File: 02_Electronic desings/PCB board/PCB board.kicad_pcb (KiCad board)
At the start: 2 copper layers, 131.6 x 84.8 mm, 31 parts, among them J10 Switch Manual/Auto, J11 Jetson, J12 Compass, J15 M2_Controll, J16 Power +5V, J17 GPS, J18 Power +5V, J19 Power +5V, J20 I2C, J21 Power +5V, J22 XBee, J3 Power +5V, J4 M1 encoder, J5 PS2_Controll, J6 M2 encoder, J8 Arduino_Mega_Header, J9 M1_Controll, U3 Logic_Level_Converter, U4 Screw_term_p2_5mm

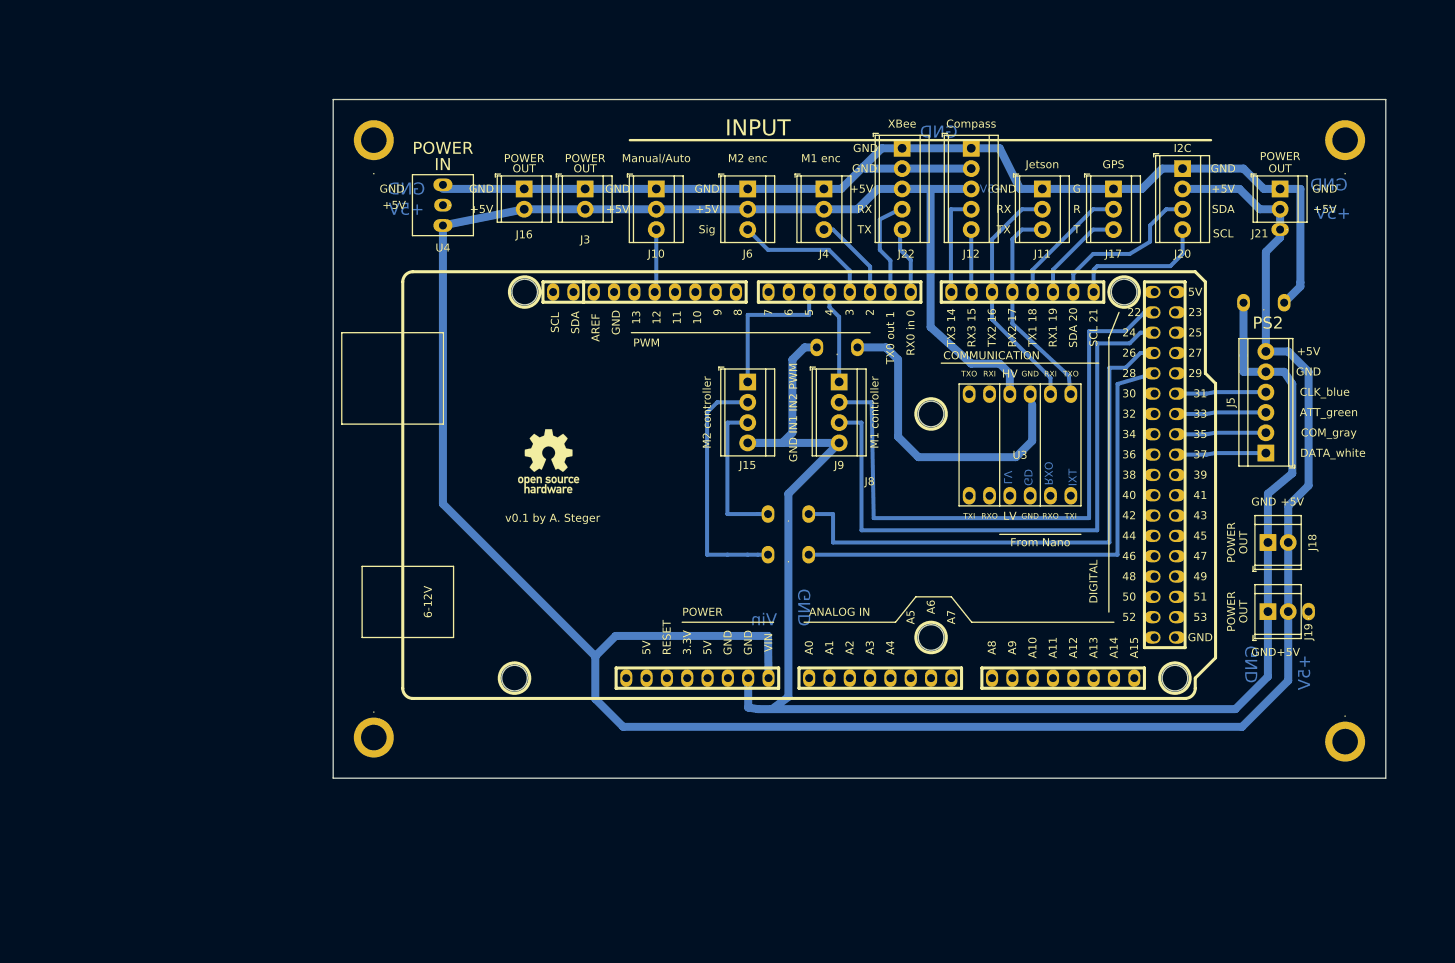
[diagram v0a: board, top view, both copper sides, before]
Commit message: Upade
new version
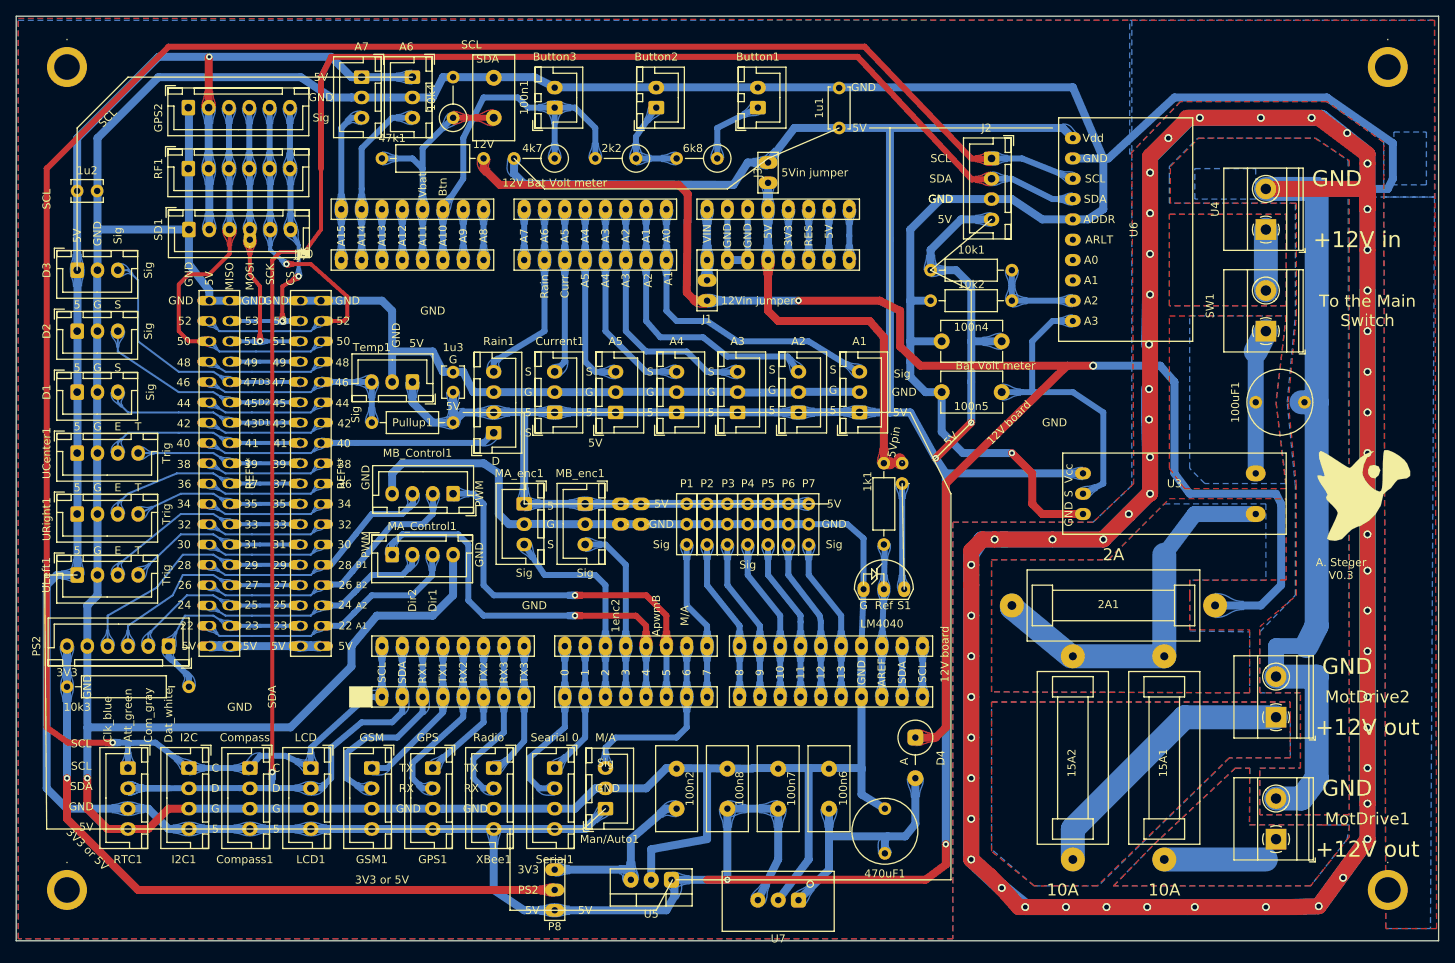
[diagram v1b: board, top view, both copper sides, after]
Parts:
- removed the . at (209.8, 111.3)
- removed the . at (214.4, 127.5)
- removed the . at (214.4, 52.3)
- removed the . at (206.2, 63.5)
- removed the . at (101.6, 60.5)
- removed the . at (204.2, 72.6)
- removed the . at (150.9, 78.2)
- removed the . at (144.8, 104.1)
- removed the . at (144.8, 99.1)
- removed the . at (93.0, 52.3)
- removed the . at (93.0, 127.0)
- removed J12: Compass, TerminalBlock_TE-Connectivity:TerminalBlock_TE_282834-5_1x05_P2.54mm_Horizontal
- removed J20: I2C, TerminalBlock_TE-Connectivity:TerminalBlock_TE_282834-4_1x04_P2.54mm_Horizontal
- removed J21: Power +5V, TerminalBlock_TE-Connectivity:TerminalBlock_TE_282834-2_1x02_P2.54mm_Horizontal
- removed J22: XBee, TerminalBlock_TE-Connectivity:TerminalBlock_TE_282834-5_1x05_P2.54mm_Horizontal
- removed J4: M1 encoder, TerminalBlock_TE-Connectivity:TerminalBlock_TE_282834-3_1x03_P2.54mm_Horizontal
- removed J8: Arduino_Mega_Header, Arduino:Arduino_MEGA
- removed the REF** at (114.8, 92.5)
- added .: ., Arduino:1_pin, F.Cu at (77.5, 64.8)
- added .: 1pin, Arduino:1pin, F.Cu at (219.7, 146.1)
- added .: 1pin, Arduino:1pin, F.Cu at (54.6, 146.1)
- added .: ., Arduino:1_pin, F.Cu at (126.4, 100.3)
- added .: ., Arduino:1_pin, F.Cu at (123.8, 100.3)
- added .: ., Arduino:1_pin, F.Cu at (123.8, 97.8)
- added .: ., Arduino:1_pin, F.Cu at (126.4, 97.8)
- added .: ., Arduino:1_pin, F.Cu at (159.0, 92.7)
- added .: ., Arduino:1_pin, F.Cu at (159.0, 95.2)
- added .: 1pin, Arduino:1pin, F.Cu at (219.7, 43.2)
- added .: 1pin, Arduino:1pin, F.Cu at (54.6, 43.2)
- added 100n1: 100nF, Capacitor_THT:C_Disc_D10.5mm_W5.0mm_P5.00mm, F.Cu at (108.0, 49.5)
- added 100n2: 100nF, Capacitor_THT:C_Disc_D10.5mm_W5.0mm_P5.00mm, F.Cu at (130.8, 135.9)
- added 100n4: 100n, Capacitor_THT:C_Disc_D7.5mm_W5.0mm_P7.50mm, F.Cu at (171.4, 77.5)
- added 100n5: 100n, Capacitor_THT:C_Disc_D7.5mm_W5.0mm_P7.50mm, F.Cu at (171.4, 83.8)
- added 100n6: 100nF, Capacitor_THT:C_Disc_D10.5mm_W5.0mm_P5.00mm, F.Cu at (149.9, 135.9)
- added 100n7: 100nF, Capacitor_THT:C_Disc_D10.5mm_W5.0mm_P5.00mm, F.Cu at (143.5, 135.9)
- added 100n8: 100nF, Capacitor_THT:C_Disc_D10.5mm_W5.0mm_P5.00mm, F.Cu at (137.2, 135.9)
- added 100uF1: 100 uF, Capacitor_THT:C_Radial_D8.0mm_H7.0mm_P3.50mm, F.Cu at (204.5, 85.1)
- added 10k1: 10k, Resistor_THT:R_Axial_DIN0207_L6.3mm_D2.5mm_P10.16mm_Horizontal, F.Cu at (162.6, 68.6)
- added 10k2: 10k, Resistor_THT:R_Axial_DIN0207_L6.3mm_D2.5mm_P10.16mm_Horizontal, F.Cu at (172.7, 72.4)
- added 10k3: 10k, Resistor_THT:R_Axial_DIN0207_L6.3mm_D2.5mm_P10.16mm_Horizontal, F.Cu at (54.6, 120.7)
- added 10k4: 10k, Resistor_THT:R_Axial_DIN0309_L9.0mm_D3.2mm_P5.08mm_Vertical, F.Cu at (102.9, 49.5)
- added 15A1: 15A1, Shield:Fuse, F.Cu at (191.8, 129.5)
- added 15A2: 15A1, Shield:Fuse, F.Cu at (180.3, 129.5)
- added 1k1: 1k, Resistor_THT:R_Axial_DIN0207_L6.3mm_D2.5mm_P10.16mm_Horizontal, F.Cu at (156.7, 92.7)
- added 1u1: 1u, Capacitor_THT:C_Disc_D5.0mm_W2.5mm_P5.00mm, F.Cu at (151.1, 50.8)
- added 1u2: 1u, Capacitor_THT:C_Disc_D3.8mm_W2.6mm_P2.50mm, F.Cu at (55.9, 58.7)
- added 1u3: 1u, Capacitor_THT:C_Disc_D3.8mm_W2.6mm_P2.50mm, F.Cu at (102.9, 83.8)
- added 2A1: 2A, Shield:Fuse, F.Cu at (185.4, 110.5)
- added 2k2: 2k2, Resistor_THT:R_Axial_DIN0309_L9.0mm_D3.2mm_P5.08mm_Vertical, F.Cu at (125.7, 54.6)
- added 470uF1: 470uF, Capacitor_THT:C_Radial_D8.0mm_H7.0mm_P3.50mm, F.Cu at (156.8, 140.5)
- added 47k1: 47k1, Resistor_THT:R_Axial_DIN0309_L9.0mm_D3.2mm_P12.70mm_Horizontal, F.Cu at (106.7, 54.6)
- added 4k7: 4k7, Resistor_THT:R_Axial_DIN0309_L9.0mm_D3.2mm_P5.08mm_Vertical, F.Cu at (115.6, 54.6)
- added 6k8: 6k8, Resistor_THT:R_Axial_DIN0309_L9.0mm_D3.2mm_P5.08mm_Vertical, F.Cu at (135.9, 54.6)
- added A1: s1, Connector_JST:JST_XH_B3B-XH-A_1x03_P2.50mm_Vertical, F.Cu at (153.7, 86.4)
- added A2: s1, Connector_JST:JST_XH_B3B-XH-A_1x03_P2.50mm_Vertical, F.Cu at (146.1, 86.4)
- added A3: s1, Connector_JST:JST_XH_B3B-XH-A_1x03_P2.50mm_Vertical, F.Cu at (138.4, 86.4)
- added A4: s1, Connector_JST:JST_XH_B3B-XH-A_1x03_P2.50mm_Vertical, F.Cu at (130.8, 86.4)
- added A5: s1, Connector_JST:JST_XH_B3B-XH-A_1x03_P2.50mm_Vertical, F.Cu at (123.2, 86.4)
- added A6: s1, Connector_JST:JST_XH_B3B-XH-A_1x03_P2.50mm_Vertical, F.Cu at (97.8, 44.5)
- added A7: s1, Connector_JST:JST_XH_B3B-XH-A_1x03_P2.50mm_Vertical, F.Cu at (91.4, 44.5)
- added Button1: TestBtn1, Connector_JST:JST_XH_B2B-XH-A_1x02_P2.50mm_Vertical, F.Cu at (141.0, 48.3)
- added Button2: TestBtn2, Connector_JST:JST_XH_B2B-XH-A_1x02_P2.50mm_Vertical, F.Cu at (128.3, 48.3)
- added Button3: TestBtn3, Connector_JST:JST_XH_B2B-XH-A_1x02_P2.50mm_Vertical, F.Cu at (115.6, 48.3)
- added Compass1: Compass, Connector_JST:JST_XH_B4B-XH-A_1x04_P2.50mm_Vertical, F.Cu at (77.5, 130.8)
- added Current1: Current sensor, Connector_JST:JST_XH_B3B-XH-A_1x03_P2.50mm_Vertical, F.Cu at (115.6, 86.4)
- added D1: s1, Connector_JST:JST_XH_B3B-XH-A_1x03_P2.50mm_Vertical, F.Cu at (55.9, 83.8)
- added D2: s1, Connector_JST:JST_XH_B3B-XH-A_1x03_P2.50mm_Vertical, F.Cu at (55.9, 76.2)
- added D3: s1, Connector_JST:JST_XH_B3B-XH-A_1x03_P2.50mm_Vertical, F.Cu at (55.9, 68.6)
- added D4: 1N4001, Diode_THT:D_5W_P5.08mm_Vertical_AnodeUp, F.Cu at (160.7, 127.0)
- added G***: LOGO, Shield:parrot, B.Cu at (171.4, 44.5)
- added G***: LOGO, Shield:parrot, F.Cu at (216.7, 96.5)
- added GPS1: GPS, Connector_JST:JST_XH_B4B-XH-A_1x04_P2.50mm_Vertical, F.Cu at (100.3, 130.8)
- added GPS2: GSP rov, Connector_JST:JST_XH_B6B-XH-A_1x06_P2.50mm_Vertical, F.Cu at (69.8, 48.3)
- added GSM1: GSM, Connector_JST:JST_XH_B4B-XH-A_1x04_P2.50mm_Vertical, F.Cu at (92.7, 130.8)
- added I2C1: I2C, Connector_JST:JST_XH_B4B-XH-A_1x04_P2.50mm_Vertical, F.Cu at (69.8, 130.8)
- added J1: HEADER_2, Arduino:Terminal_p2, F.Cu at (134.6, 71.1)
- added J14: ., Arduino:Terminal_p10, F.Cu at (150.1, 121.9)
- added J2: ST_01x04, Connector_JST:JST_XH_B4B-XH-A_1x04_P2.50mm_Vertical, F.Cu at (170.2, 54.6)
- added J7: ., Arduino:Terminal_p8, F.Cu at (97.8, 61.0)
- added LCD1: LCD display, Connector_JST:JST_XH_B4B-XH-A_1x04_P2.50mm_Vertical, F.Cu at (85.1, 130.8)
- added MA_Control1: MA_Control, Connector_JST:JST_XH_B4B-XH-A_1x04_P2.50mm_Vertical, F.Cu at (95.2, 104.1)
- added MA_enc1: MA_enc1, Connector_JST:JST_XH_B3B-XH-A_1x03_P2.50mm_Vertical, F.Cu at (111.8, 97.8)
- added MB_Control1: MB_Control, Connector_JST:JST_XH_B4B-XH-A_1x04_P2.50mm_Vertical, F.Cu at (102.9, 96.5)
- added MB_enc1: MB encoder, Connector_JST:JST_XH_B3B-XH-A_1x03_P2.50mm_Vertical, F.Cu at (119.4, 97.8)
- added Man/Auto1: Switch Manual/Auto, Connector_JST:JST_XH_B3B-XH-A_1x03_P2.50mm_Vertical, F.Cu at (121.9, 135.9)
- added MotDrive1: 12V Mot1 OUT, TerminalBlock_Phoenix:TerminalBlock_Phoenix_MKDS-1,5-2-5.08_1x02_P5.08mm_Horizontal, F.Cu at (205.7, 139.7)
- added MotDrive2: 12V Mot2 OUT, TerminalBlock_Phoenix:TerminalBlock_Phoenix_MKDS-1,5-2-5.08_1x02_P5.08mm_Horizontal, F.Cu at (205.7, 124.5)
- added P1: HEADER_3, Arduino:Terminal_p3_sp, F.Cu at (132.1, 100.3)
- added P2: HEADER_3, Arduino:Terminal_p3_sp, F.Cu at (134.6, 100.3)
- added P3: HEADER_3, Arduino:Terminal_p3_sp, F.Cu at (137.2, 100.3)
- added P4: HEADER_3, Arduino:Terminal_p3_sp, F.Cu at (139.7, 100.3)
- added P5: HEADER_3, Arduino:Terminal_p3_sp, F.Cu at (142.2, 100.3)
- added P6: HEADER_3, Arduino:Terminal_p3_sp, F.Cu at (144.8, 100.3)
- added P7: HEADER_3, Arduino:Terminal_p3_sp, F.Cu at (147.3, 100.3)
- added P8: HEADER_3, Arduino:Terminal_p3, F.Cu at (115.6, 146.1)
- added PS2: PS2_Controll, Connector_JST:JST_XH_B6B-XH-A_1x06_P2.50mm_Vertical, F.Cu at (67.3, 115.6)
- added Pullup1: 4k7, Resistor_THT:R_Axial_DIN0207_L6.3mm_D2.5mm_P10.16mm_Horizontal, F.Cu at (102.9, 87.6)
- added REF**: Terminal_p36, Arduino:Terminal_p36, F.Cu at (74.9, 94.0)
- added REF**: Terminal_p36, Arduino:Terminal_p36, F.Cu at (86.4, 94.0)
- added RF1: RF rov, Connector_JST:JST_XH_B6B-XH-A_1x06_P2.50mm_Vertical, F.Cu at (69.8, 55.9)
- added RTC1: RTC, Connector_JST:JST_XH_B4B-XH-A_1x04_P2.50mm_Vertical, F.Cu at (62.2, 130.8)
- added Rain1: Rain Sensor, Connector_JST:JST_XH_B4B-XH-A_1x04_P2.50mm_Vertical, F.Cu at (108.0, 88.9)
- added S1: LM4040 2.5V, Arduino:TO-92, F.Cu at (156.7, 108.5)
- added SD1: SD card, Connector_JST:JST_XH_B6B-XH-A_1x06_P2.50mm_Vertical, F.Cu at (69.8, 63.5)
- added SW1: SW_DIP_x01, TerminalBlock_Phoenix:TerminalBlock_Phoenix_MKDS-1,5-2-5.08_1x02_P5.08mm_Horizontal, F.Cu at (204.5, 76.2)
- added Serial1: Serial 0, Connector_JST:JST_XH_B4B-XH-A_1x04_P2.50mm_Vertical, F.Cu at (115.6, 130.8)
- added Temp1: Temp sensor, Connector_JST:JST_XH_B3B-XH-A_1x03_P2.50mm_Vertical, F.Cu at (97.8, 82.5)
- added U5: LM7803_TO220, Package_TO_SOT_THT:TO-220-3_Vertical, F.Cu at (130.2, 144.8)
- added U6: ADS1115, Arduino:ADS1115, F.Cu at (185.4, 63.5)
- added U7: LM7805_TO220, My_footprint_library:Traco_TSR2, F.Cu at (143.5, 147.3)
- added UCenter1: Ultrason_Right, Connector_JST:JST_XH_B4B-XH-A_1x04_P2.50mm_Vertical, F.Cu at (55.9, 91.4)
- added ULeft1: Ultrasonic Left, Connector_JST:JST_XH_B4B-XH-A_1x04_P2.50mm_Vertical, F.Cu at (55.9, 106.7)
- added URight1: Ultrason_Right, Connector_JST:JST_XH_B4B-XH-A_1x04_P2.50mm_Vertical, F.Cu at (55.9, 99.1)
- added XBee1: XBee, Connector_JST:JST_XH_B4B-XH-A_1x04_P2.50mm_Vertical, F.Cu at (108.0, 130.8)
- J10: value Switch Manual/Auto -> .; footprint TerminalBlock_TE-Connectivity:TerminalBlock_TE_282834-3_1x03_P2.54mm_Horizontal -> Arduino:Terminal_p8
- J11: value Jetson -> .; footprint TerminalBlock_TE-Connectivity:TerminalBlock_TE_282834-3_1x03_P2.54mm_Horizontal -> Arduino:Terminal_p8
- J15: value M2_Controll -> .; footprint TerminalBlock_TE-Connectivity:TerminalBlock_TE_282834-4_1x04_P2.54mm_Horizontal -> Arduino:Terminal_p8
- J16, J18, J19: value Power +5V -> .; footprint TerminalBlock_TE-Connectivity:TerminalBlock_TE_282834-2_1x02_P2.54mm_Horizontal -> Arduino:Terminal_p8
- J17: value GPS -> .; footprint TerminalBlock_TE-Connectivity:TerminalBlock_TE_282834-3_1x03_P2.54mm_Horizontal -> Arduino:Terminal_p10
- J3: value Power +5V -> HEADER_2; footprint TerminalBlock_TE-Connectivity:TerminalBlock_TE_282834-2_1x02_P2.54mm_Horizontal -> Arduino:Terminal_p2
- J5: value PS2_Controll -> .; footprint TerminalBlock_TE-Connectivity:TerminalBlock_TE_282834-6_1x06_P2.54mm_Horizontal -> Arduino:Terminal_p8
- J6: value M2 encoder -> .; footprint TerminalBlock_TE-Connectivity:TerminalBlock_TE_282834-3_1x03_P2.54mm_Horizontal -> Arduino:Terminal_p8
- J9: value M1_Controll -> .; footprint TerminalBlock_TE-Connectivity:TerminalBlock_TE_282834-4_1x04_P2.54mm_Horizontal -> Arduino:Terminal_p8
- U3: value Logic_Level_Converter -> ACS712_30A; footprint Arduino:Logic_Level_Converter -> My_footprint_library:ASC712
- U4: value Screw_term_p2_5mm -> ST; footprint Arduino:Screw_term_p2_5mm -> TerminalBlock_Phoenix:TerminalBlock_Phoenix_MKDS-1,5-2-5.08_1x02_P5.08mm_Horizontal
- moved U4 102.9 mm to (204.5, 63.5)
- moved J19 101.9 mm to (102.9, 115.6)
- moved J18 80.0 mm to (125.7, 115.6)
- moved J11 79.2 mm to (97.8, 67.3), turned to 180 degrees
- moved J17 67.2 mm to (150.1, 115.6), turned to 0 degrees
- moved J5 65.6 mm to (143.5, 67.3), turned to 180 degrees
- moved J16 64.1 mm to (102.9, 121.9), turned to 0 degrees
- moved J15 41.8 mm to (125.7, 121.9), turned to 0 degrees
- moved J3 23.0 mm to (142.2, 56.4), turned to 90 degrees
- moved J9 22.9 mm to (143.5, 61.0), turned to 180 degrees
- moved J6 21.0 mm to (120.7, 67.3), turned to 180 degrees
- moved U3 20.2 mm to (193.0, 96.5), turned to 180 degrees
- moved J10 8.03 mm to (120.7, 61.0), turned to 180 degrees
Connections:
- J10 pad 1: GND -> /A1
- J10 pad 2: +5V -> /A2
- J10 pad 3: Net-(J10-Pad3) -> /A3
- J11 pad 1: GND -> Net-(J11-Pad1)
- J11 pad 2: /RX -> Net-(J11-Pad2)
- J11 pad 3: /TX -> /Button
- J15 pad 1: Net-(J15-Pad1) -> /RX0
- J15 pad 2: Net-(J15-Pad2) -> /TX0
- J15 pad 3: Net-(J15-Pad3) -> /M1Enc
- J15 pad 4: GND -> /M2Enc
- J16 pad 1: GND -> /SCL
- J16 pad 2: +5V -> /SDA
- J17 pad 1: GND -> /PWM_2
- J17 pad 2: Net-(J17-Pad2) -> /PWM_3
- J17 pad 3: Net-(J17-Pad3) -> /PWM_4
- J18 pad 1: GND -> /RX0
- J18 pad 2: +5V -> /TX0
- J19 pad 1: GND -> /SCL
- J19 pad 2: +5V -> /SDA
- J3 pad 1: GND -> /5Vpin
- J3 pad 2: +5V -> +5P
- J5 pad 5: GND -> /5Vpin
- J5 pad 6: +5V -> GND
- J6 pad 1: GND -> /A1
- J6 pad 2: +5V -> /A2
- J6 pad 3: Net-(J6-Pad3) -> /A3
- J9 pad 1: Net-(J8-Pad73) -> Net-(J5-Pad1)
- J9 pad 2: Net-(J8-Pad41) -> Net-(J5-Pad2)
- J9 pad 3: Net-(J8-Pad40) -> Net-(J5-Pad3)
- J9 pad 4: GND -> Net-(J5-Pad4)
- U3 pad 1: Net-(U3-Pad1) -> /CurA
- U3 pad 2: Net-(U3-Pad2) -> /CurB
- U3 pad 3: +5V -> Net-(100n5-Pad1)
- U3 pad 4: GND -> +5P
- U3 pad 5: /RX -> GND
- U4 pad 1: +5V -> Net-(SW1-Pad2)
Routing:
- net GND: track 332.4 -> 1627.8 mm, vias 0 -> 55
- net +5P: track 0.00 -> 673.5 mm, vias 0 -> 5
- net +5V: track 366.6 -> 0.00 mm
- net /SCL: track 0.00 -> 270.4 mm, vias 0 -> 1
- net /SDA: track 0.00 -> 252.5 mm, vias 0 -> 1
- net +12V: track 0.00 -> 210.4 mm, vias 0 -> 2
- net (no net): track 38.6 -> 186.4 mm, vias 0 -> 1
- net Net-(J15-Pad2): track 95.3 -> 0.00 mm
- net Net-(J15-Pad3): track 88.5 -> 0.00 mm
- net Net-(10k3-Pad1): track 0.00 -> 86.2 mm, vias 0 -> 1
- net Net-(J8-Pad41): track 78.0 -> 0.00 mm
- net Net-(J8-Pad40): track 76.8 -> 0.00 mm
- net /RX: track 56.5 -> 0.00 mm
- net /MISO: track 0.00 -> 51.3 mm
- net /PWM_A: track 0.00 -> 51.3 mm, vias 0 -> 1
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- added copper zone on B.Cu, net (none)
- added copper zone on B.Cu, net /CurA
- added copper zone on F.Cu, net /CurA
- added copper zone on B.Cu, net /CurB
- added copper zone on F.Cu, net /CurB
- added copper zone on B.Cu, net GND
- added copper zone on F.Cu, net GND
- added copper zone on B.Cu, net Net-(15A1-Pad2)
- added copper zone on F.Cu, net Net-(15A1-Pad2)
- added copper zone on B.Cu, net Net-(15A2-Pad2)
- added copper zone on F.Cu, net Net-(15A2-Pad2)
- added copper zone on B.Cu, net Net-(SW1-Pad2)
- added copper zone on F.Cu, net Net-(SW1-Pad2)
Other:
- board size 131.6 x 84.8 mm -> 177.8 x 115.6 mm
- net class PWR+GND added: clearance 0.4, trace_width 1, via_dia 0.8, via_drill 0.4
- board text added: "+12V"
- board text added: "+12V in"
- board text added: "+12V out"
- board text added: "0"
- board text added: "1"
- board text added: "10"
- board text added: "100n"
- board text added: "10A"
- board text added: "10k"
- board text added: "11"
- board text added: "12"
- board text added: "12V"
- board text added: "12V Bat Volt meter"
- board text added: "12V board"
- board text added: "12V in"
- board text added: "12V out"
- board text added: "12Vin jumper"
- board text added: "13"
- board text added: "1enc2"
- board text added: "1k"
- board text added: "1u"
- board text added: "2"
- board text added: "22"
- board text added: "23"
- board text added: "24"
- board text added: "25"
- board text added: "26"
- board text added: "27"
- board text added: "28"
- board text added: "29"
- board text added: "2A"
- board text added: "2k2"
- board text added: "3"
- board text added: "30"
- board text added: "31"
- board text added: "32"
- board text added: "33"
- board text added: "34"
- board text added: "35"
- board text added: "36"
- board text added: "37"
- board text added: "38"
- board text added: "39"
- board text added: "3V3"
- board text added: "3V3 or 5V"
- board text added: "4"
- board text added: "40"
- board text added: "41"
- board text added: "42"
- board text added: "43"
- board text added: "44"
- board text added: "45"
- board text added: "46"
- board text added: "47"
- board text added: "470u"
- board text added: "47k"
- board text added: "48"
- board text added: "49"
- board text added: "4k7"
- board text added: "5"
- board text added: "50"
- board text added: "51"
- board text added: "52"
- board text added: "53"
- board text added: "5V"
- board text added: "5V supply"
- board text added: "5Vin jumper"
- board text added: "5Vpin"
- board text added: "6"
- board text added: "6k8"
- board text added: "7"
- board text added: "8"
- board text added: "9"
- board text added: "A. Steger V0.3"
- board text added: "A0"
- board text added: "A1"
- board text added: "A10"
- board text added: "A11"
- board text added: "A12"
- board text added: "A13"
- board text added: "A14"
- board text added: "A15"
- board text added: "A2"
- board text added: "A3"
- board text added: "A4"
- board text added: "A5"
- board text added: "A6"
- board text added: "A7"
- board text added: "A8"
- board text added: "A9"
- board text added: "ADDR"
- board text added: "ALRT"
- board text added: "AREF"
- board text added: "ATT"
- board text added: "ApwmB"
- board text added: "Att_green"
- board text added: "B1"
- board text added: "B2"
- board text added: "Bat Volt meter"
- board text added: "Btn"
- board text added: "Button 1"
- board text added: "Button 2"
- board text added: "Button 3"
- board text added: "C"
- board text added: "CLK"
- board text added: "COM"
- board text added: "CS"
- board text added: "Cap"
- board text added: "Clk_blue"
- board text added: "Com_gray"
- board text added: "Curr"
- board text added: "Current"
- board text added: "D"
- board text added: "D1"
- board text added: "D2"
- board text added: "D3"
- board text added: "DATA"
- board text added: "Dat_white"
- board text added: "Dir A1"
- board text added: "Dir A2"
- board text added: "Dir B1"
- board text added: "Dir B2"
- board text added: "Dir1"
- board text added: "Dir2"
- board text added: "E"
- board text added: "Echo"
- board text added: "Fuse 10A"
- board text added: "Fuse 2A"
- board text added: "GSM"
- board text added: "LCD"
- board text added: "LM4040"
- board text added: "M/A"
- board text added: "MA control"
- board text added: "MB control"
- board text added: "MISO"
- board text added: "MOSI"
- board text added: "Mot drive 1"
- board text added: "Mot drive 2"
- board text added: "PWM"
- board text added: "PWM A"
- board text added: "PWM B"
- board text added: "RES"
- board text added: "RTC"
- board text added: "RX1"
- board text added: "RX2"
- board text added: "RX3"
- board text added: "Radio"
- board text added: "Rain"
- board text added: "RainA"
- board text added: "RainD"
- board text added: "S"
- board text added: "SCK"
- board text added: "Searial 0"
- board text added: "Serial 0"
- board text added: "Switch"
- board text added: "TX1"
- board text added: "TX2"
- board text added: "TX3"
- board text added: "Temp"
- board text added: "To the Main Switch"
- board text added: "Trig"
- board text added: "UCenter"
- board text added: "ULeft"
- board text added: "URight"
- board text added: "VIN"
- board text added: "Vbat"
- board text added: "current met"
- board text added: "diode"
- board text removed: "+5V"
- board text removed: "ATT_green"
- board text removed: "CLK_blue"
- board text removed: "COM_gray"
- board text removed: "DATA_white"
- board text removed: "From Nano"
- board text removed: "GD"
- board text removed: "GND IN1 IN2 PWM"
- board text removed: "IN"
- board text removed: "INPUT"
- board text removed: "Jetson"
- board text removed: "LV"
- board text removed: "M1 controller"
- board text removed: "M1 enc"
- board text removed: "M2 controller"
- board text removed: "M2 enc"
- board text removed: "Manual/Auto"
- board text removed: "OUT"
- board text removed: "POWER"
- board text removed: "R"
- board text removed: "RXO"
- board text removed: "TXI"
- board text removed: "Vin"
- board text removed: "XBee"
- board text removed: "v0.1 by A. Steger"
